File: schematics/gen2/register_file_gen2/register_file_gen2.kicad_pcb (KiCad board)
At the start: 2 copper layers, 100 x 91.1 mm, 15 parts, among them U1 74LS02, U2 74LS02

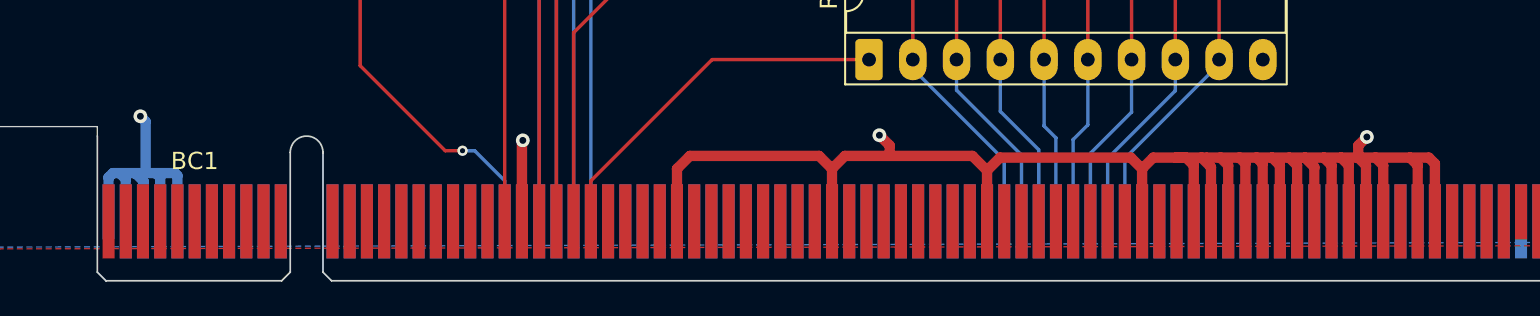
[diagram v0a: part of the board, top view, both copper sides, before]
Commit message: fixed errors
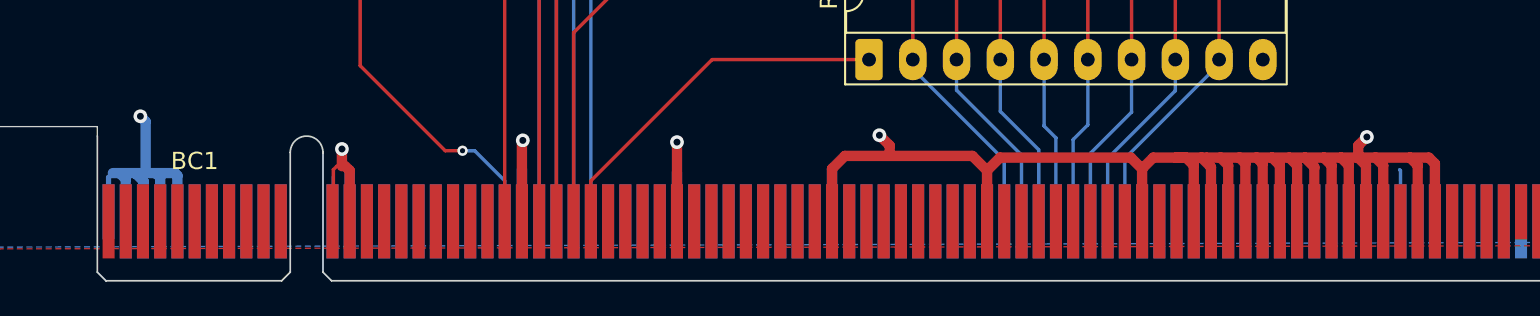
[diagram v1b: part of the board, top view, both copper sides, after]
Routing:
- net GND: track 120.4 -> 173.1 mm, vias 3 -> 5
